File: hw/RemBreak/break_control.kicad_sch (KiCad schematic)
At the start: 19 parts, among them J1 Conn_01x04, J2 Conn_01x07, J3 Screw_Terminal_01x02, J4 Conn_01x07, J5 Conn_01x03, J6 Conn_01x03, J7 Conn_01x07, J8 Conn_01x04, Q1 BC337, Q2 BC847

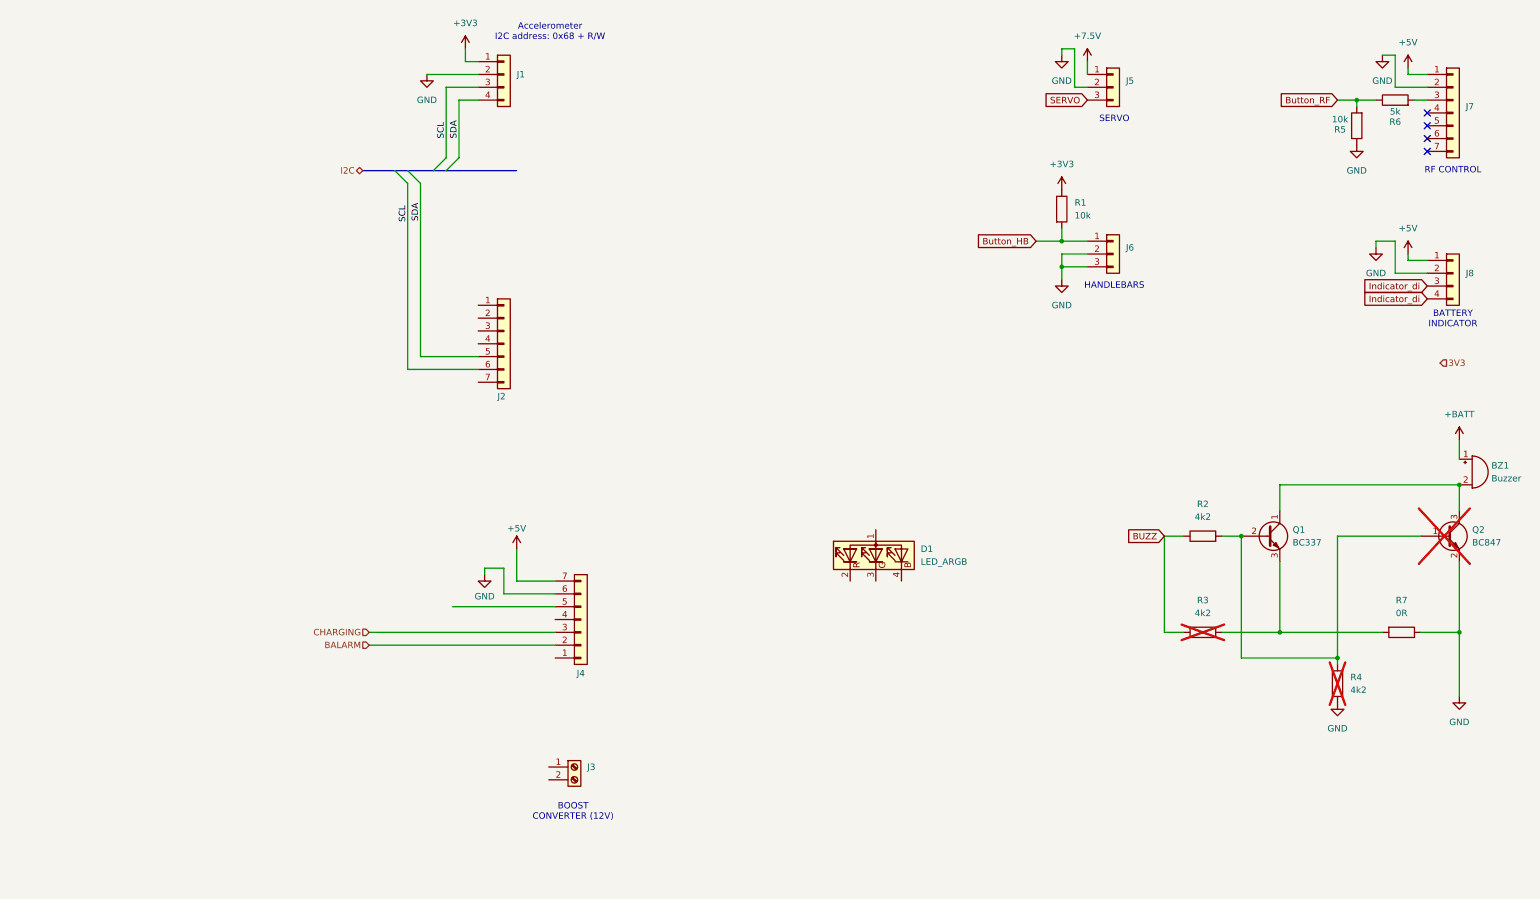
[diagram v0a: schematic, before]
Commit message: schematics drawing in progress
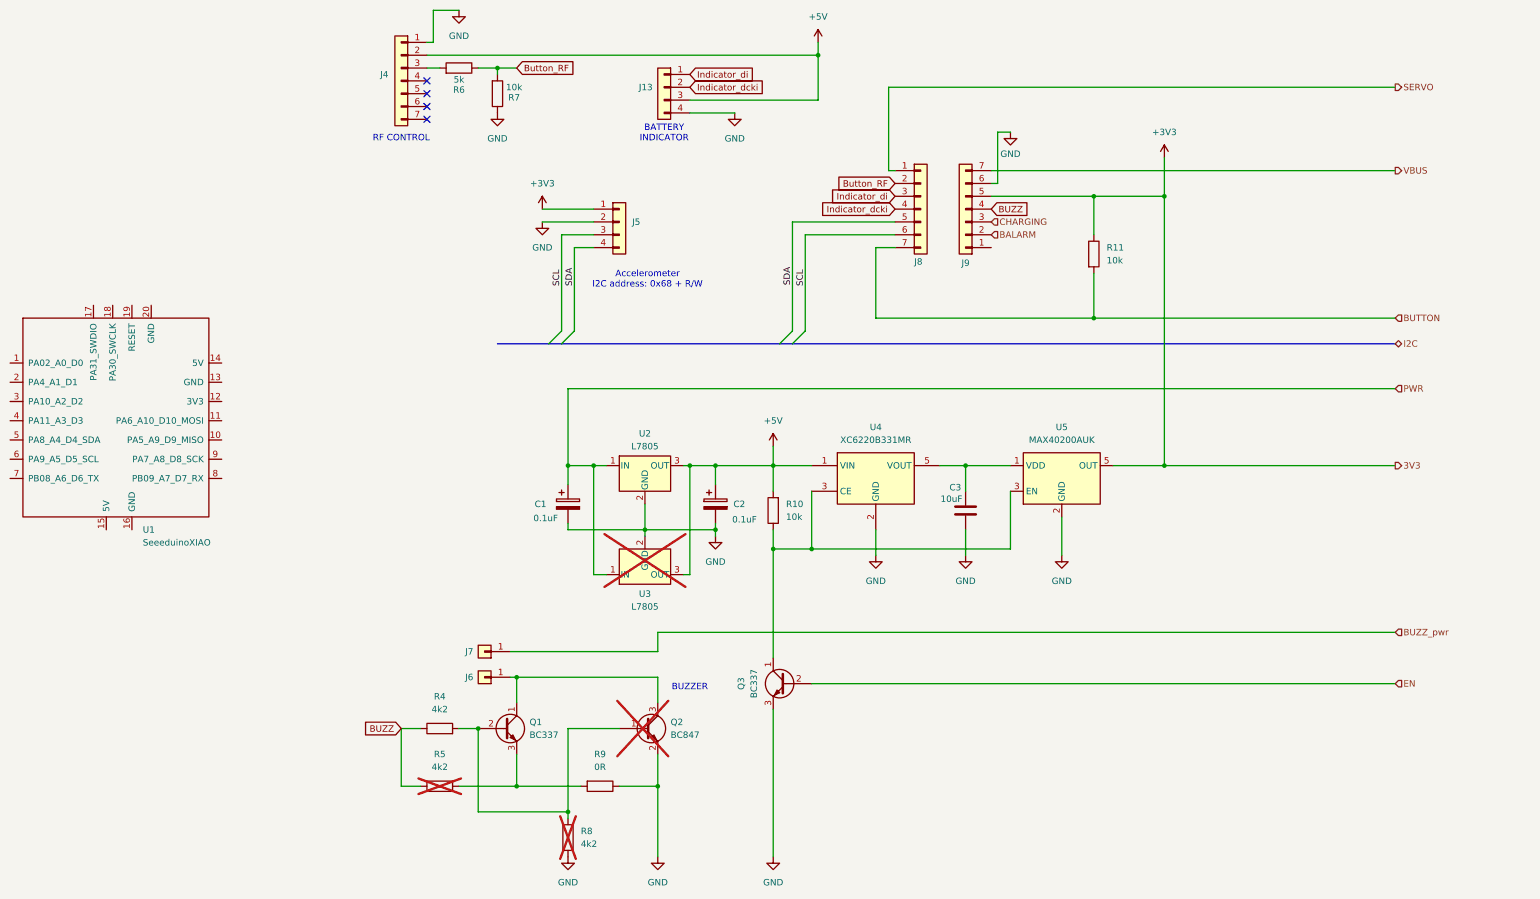
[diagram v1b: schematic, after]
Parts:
- removed BZ1: Buzzer, Buzzer_Beeper:Buzzer_12x9.5RM7.6, symbol Device:Buzzer
- removed D1: LED_ARGB, LED_SMD:LED_WS2812B-Mini_PLCC4_3.5x3.5mm, symbol Device:LED_ARGB
- removed J3: Screw_Terminal_01x02, TerminalBlock_Phoenix:TerminalBlock_Phoenix_MKDS-1,5-2_1x02_P5.00mm_Horizontal, symbol Connector:Screw_Terminal_01x02
- removed J5: Conn_01x03, Connector_PinHeader_2.54mm:PinHeader_1x03_P2.54mm_Vertical, symbol Connector_Generic:Conn_01x03
- removed J6: Conn_01x03, TerminalBlock_Phoenix:TerminalBlock_Phoenix_MKDS-1,5-2_1x02_P5.00mm_Horizontal, symbol Connector_Generic:Conn_01x03
- removed J8: Conn_01x04, Connector_Molex:Molex_KK-254_AE-6410-04A_1x04_P2.54mm_Vertical, symbol Connector_Generic:Conn_01x04
- removed R1: 10k, Resistor_SMD:R_0805_2012Metric, symbol Device:R
- added C1, C2: 0.1uF, Capacitor_SMD:C_0805_2012Metric, symbol Device:C_Polarized
- added C3: 10uF, Capacitor_SMD:C_0805_2012Metric, symbol Device:C
- added J13: Conn_01x04, Connector_PinSocket_2.54mm:PinSocket_1x04_P2.54mm_Vertical, symbol Connector_Generic:Conn_01x04
- added J6, J7: Conn_01x01, TestPoint:TestPoint_Pad_2.5x2.5mm, symbol Connector_Generic:Conn_01x01
- added Q3: BC337, Package_TO_SOT_THT:TO-92_Inline, symbol Transistor_BJT:BC337
- added R10, R11: 10k, Resistor_SMD:R_0805_2012Metric, symbol Device:R
- added U1: SeeeduinoXIAO, chinese_modules:Seeeduino XIAO-MOUDLE14P-2.54-21X17.8MM, symbol chinese_modules:SeeeduinoXIAO
- added U2: L7805, Package_TO_SOT_SMD:TO-263-2, symbol Regulator_Linear:L7805
- added U3: L7805, Package_TO_SOT_THT:TO-220-3_Horizontal_TabDown, symbol Regulator_Linear:L7805
- added U4: XC6220B331MR, Package_TO_SOT_SMD:SOT-23-5, symbol Regulator_Linear:XC6220B331MR
- added U5: MAX40200AUK, Package_TO_SOT_SMD:SOT-23-5, symbol Analog_Switch:MAX40200AUK
- renumbered J7 to J4, J1 to J5, J2 to J8, J4 to J9, R2 to R4, R3 to R5, R5 to R7, R4 to R8, R7 to R9
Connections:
- net +3V3: now also J9.5 (Pin_5), R11.1, U5.5 (OUT)
- net +5V: now also J4.2 (Pin_2), C2.1, J13.3 (Pin_3), R10.2, U2.3 (OUT), U3.3 (OUT), U4.1 (VIN); no longer J4.1 (Pin_1), J9.7 (Pin_7)
- net BUZZ: now also J9.4 (Pin_4)
- net Button_RF: now also J8.2 (Pin_2)
- net GND: now also J4.1 (Pin_1), C1.2, C2.2, C3.2, J13.4 (Pin_4), Q3.3 (E), U2.2 (GND), U3.2 (GND), U4.2 (GND), U5.2 (GND); no longer J4.2 (Pin_2)
- net Indicator_di: now also J8.3 (Pin_3), J13.1 (Pin_1)
- net SERVO: now also J8.1 (Pin_1)
- net at Q1.1 (C), Q2.3 (C): now also J6.1 (Pin_1)
- net Indicator_dcki: now reaches J8.4 (Pin_4)
- net Indicator_dcki: now also J13.2 (Pin_2)
- net BUTTON: now reaches J8.7 (Pin_7)
- net BUTTON: now also R11.2
- new net: Q3.1 (C), R10.1, U4.3 (CE), U5.3 (EN)
- new net: C3.1, U4.5 (VOUT), U5.1 (VDD)
- new net BUZZ_pwr: J7.1 (Pin_1)
- new net EN: Q3.2 (B)
- new net PWR: C1.1, U2.1 (IN), U3.1 (IN)
- new net VBUS: J9.7 (Pin_7)
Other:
- note added: "BUZZER"
- note removed: "BOOST CONVERTER (12V)"
- note removed: "HANDLEBARS"
- note removed: "SERVO"
- moved on the sheet: J4, J5, J8, J9, Q1, Q2, R4, R5, R6, R7, R8, R9
